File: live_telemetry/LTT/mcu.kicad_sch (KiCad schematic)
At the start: 15 parts, among them J1 Programming Header, U1 MC2562, U2 PIC18F26K83, Y1 Crystal

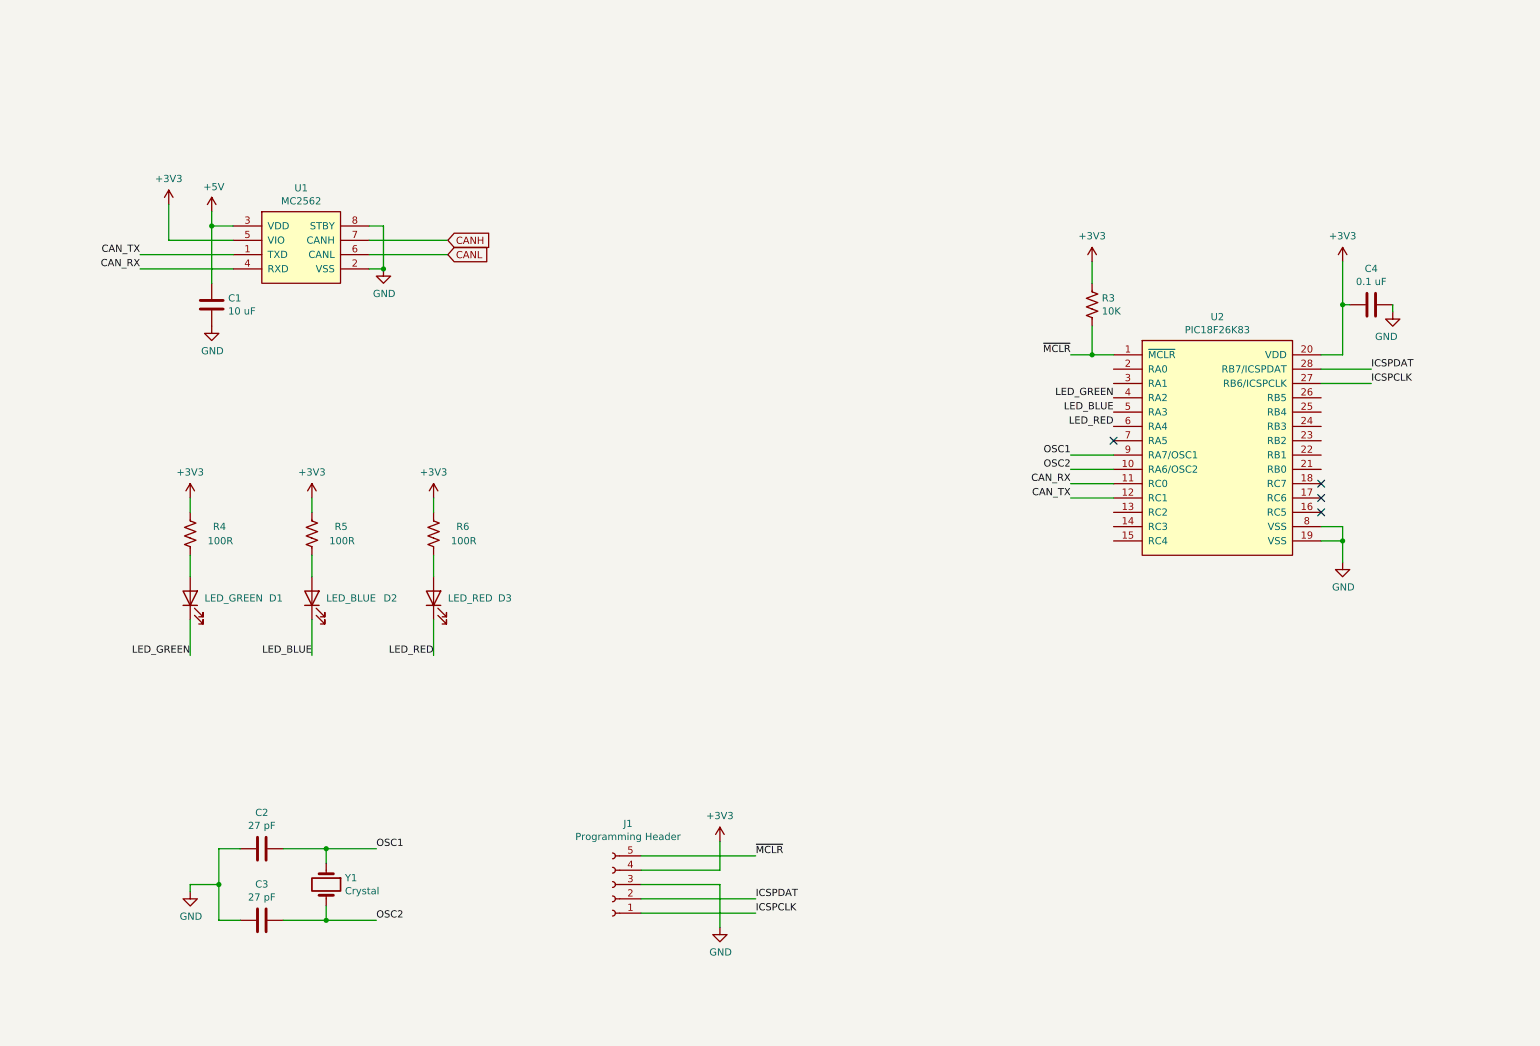
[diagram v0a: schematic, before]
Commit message: started schematic
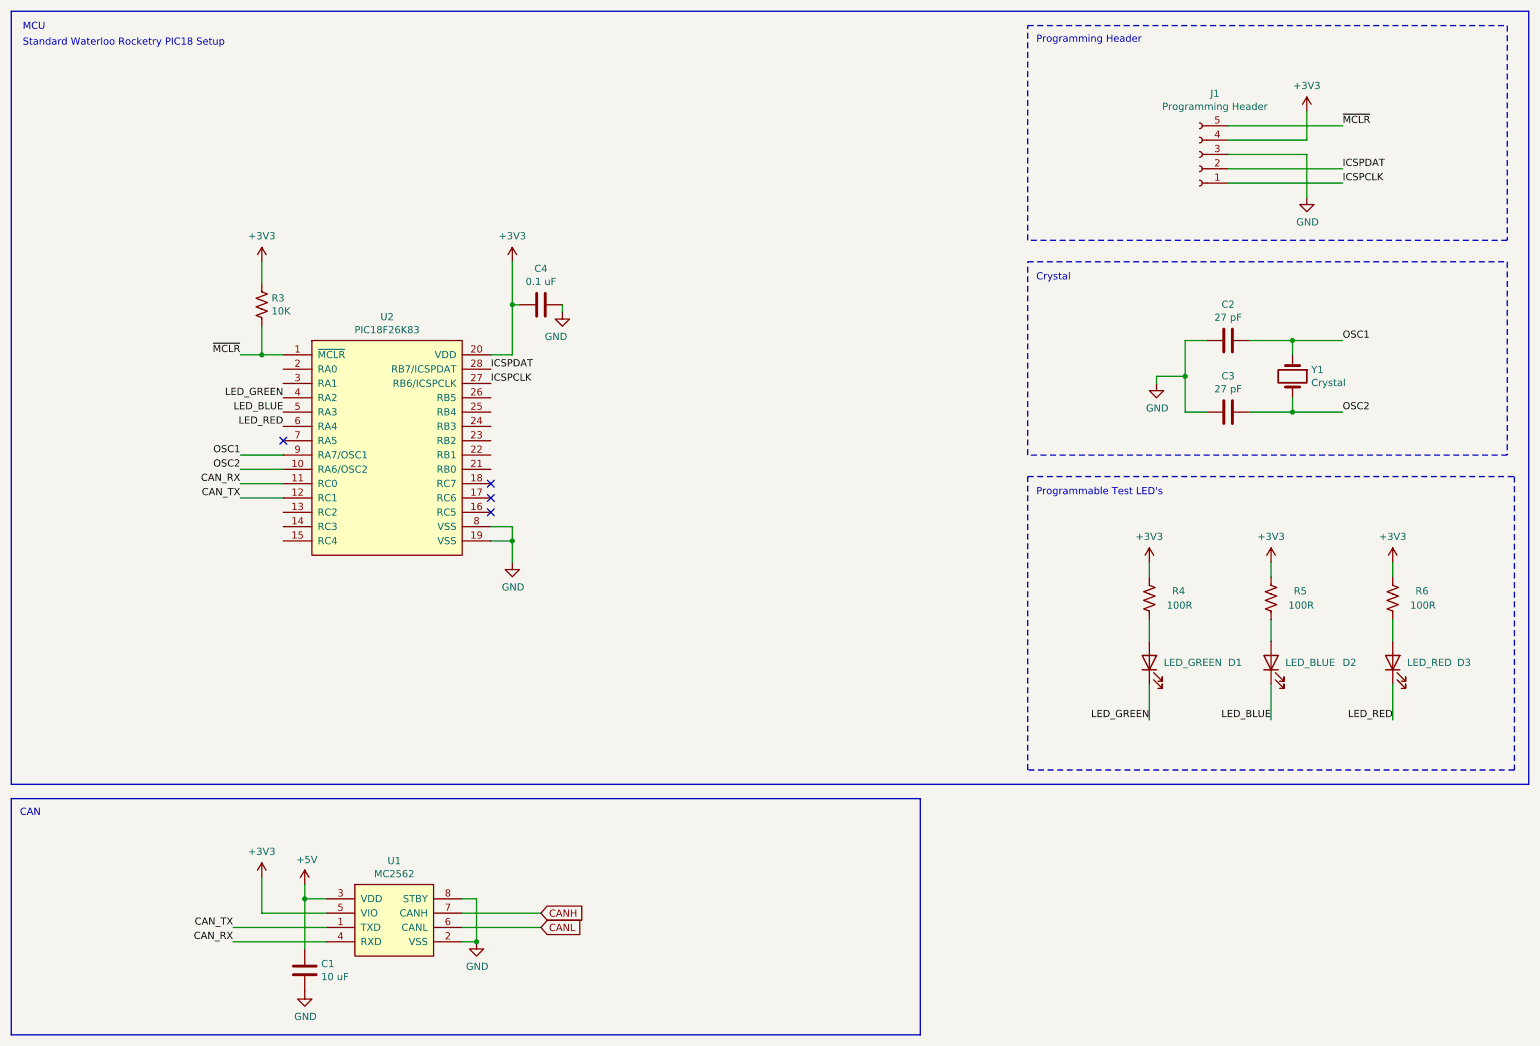
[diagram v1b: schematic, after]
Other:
- note added: "CAN"
- note added: "Crystal"
- note added: "MCU"
- note added: "Programmable Test LED's"
- note added: "Programming Header"
- note added: "Standard Waterloo Rocketry PIC18 Setup"
- moved on the sheet: C1, C2, C3, C4, D1, D2, D3, J1, R3, R4, R5, R6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
